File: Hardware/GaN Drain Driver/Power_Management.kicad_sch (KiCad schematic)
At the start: 40 parts, among them J3 0022272021, J4 0022272021, U2 LM393, U3 L7815, U4 R1SE, U5 L7805, U6 REF5040, U7 TLV9302

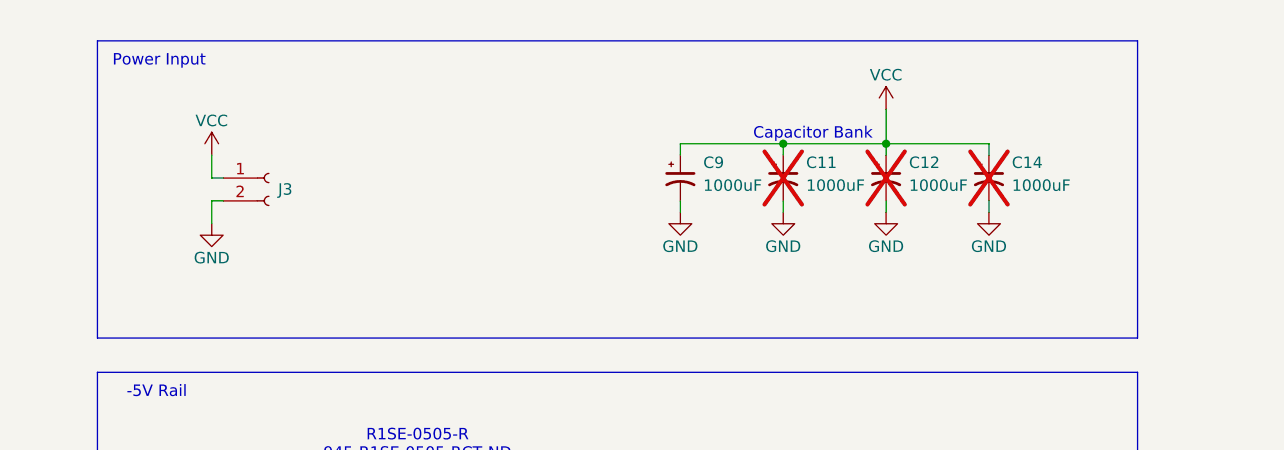
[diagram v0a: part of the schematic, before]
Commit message: Adding notes to schematic
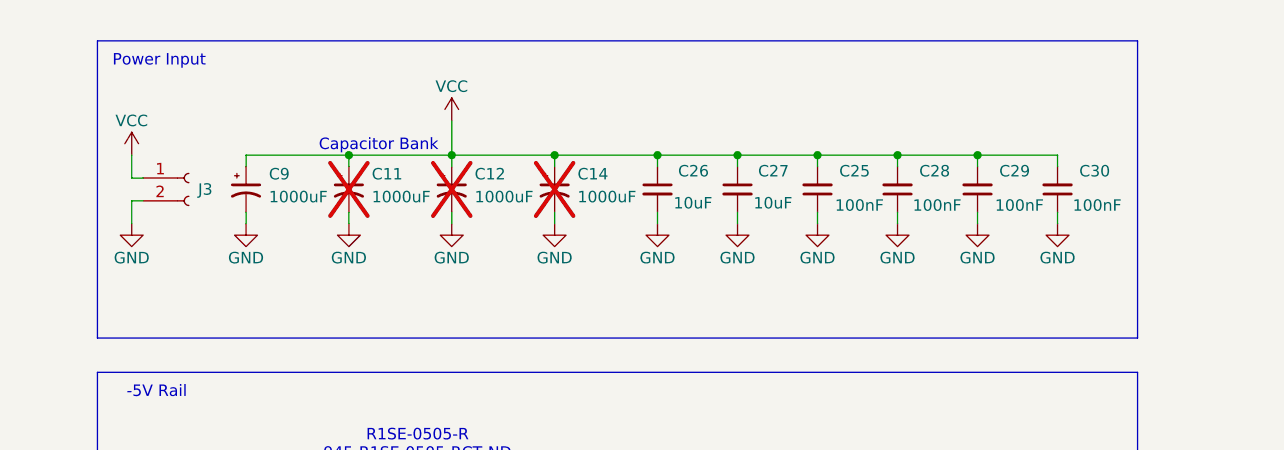
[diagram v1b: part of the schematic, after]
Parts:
- added C25, C28, C29, C30: 100nF, Capacitor_SMD:C_0805_2012Metric, symbol Device:C_Small
- added C26, C27: 10uF, Capacitor_SMD:C_0805_2012Metric, symbol Device:C_Small
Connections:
- net GND: now also C25.1, C26.2, C27.2, C28.1, C29.1, C30.1
- net VCC: now also C25.2, C26.1, C27.1, C28.2, C29.2, C30.2
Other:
- moved on the sheet: C11, C12, C14, C9, J3
